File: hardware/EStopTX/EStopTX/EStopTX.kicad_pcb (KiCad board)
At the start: 2 copper layers, 75 x 59 mm, 11 parts

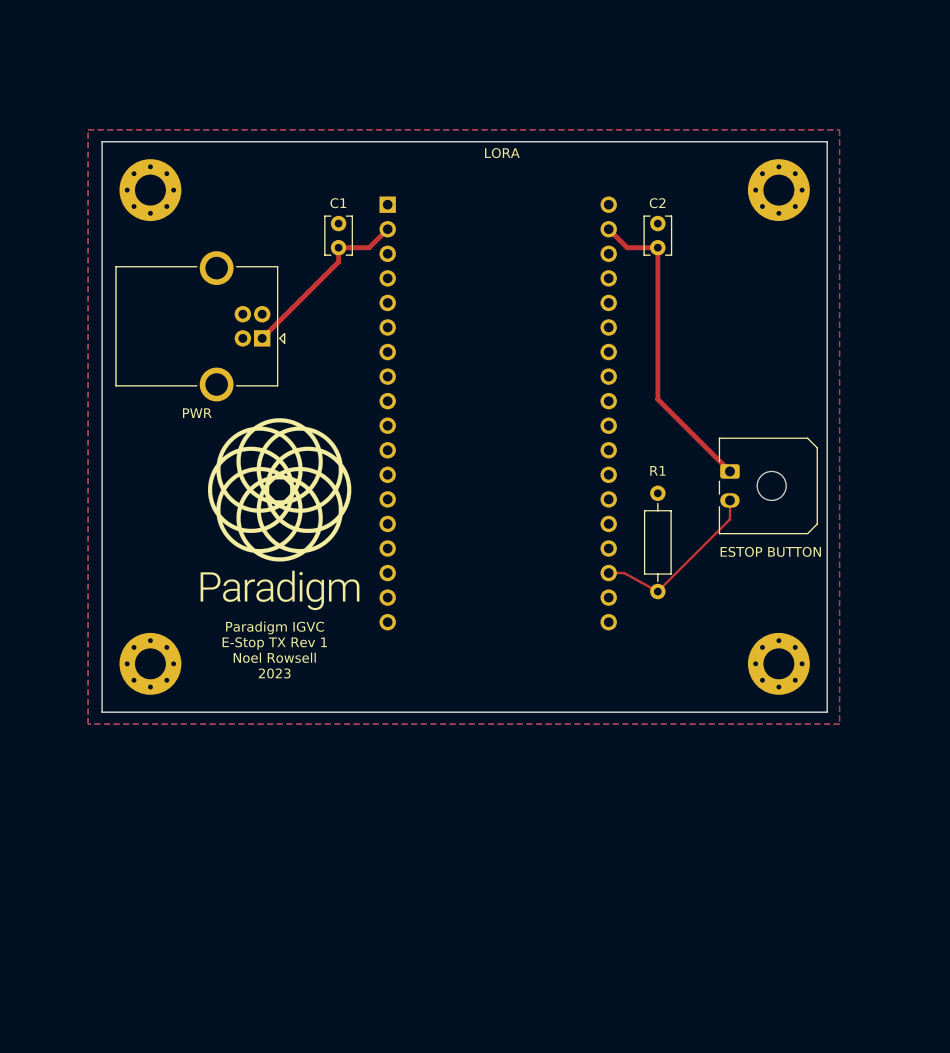
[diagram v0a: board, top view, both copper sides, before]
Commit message: adjustments
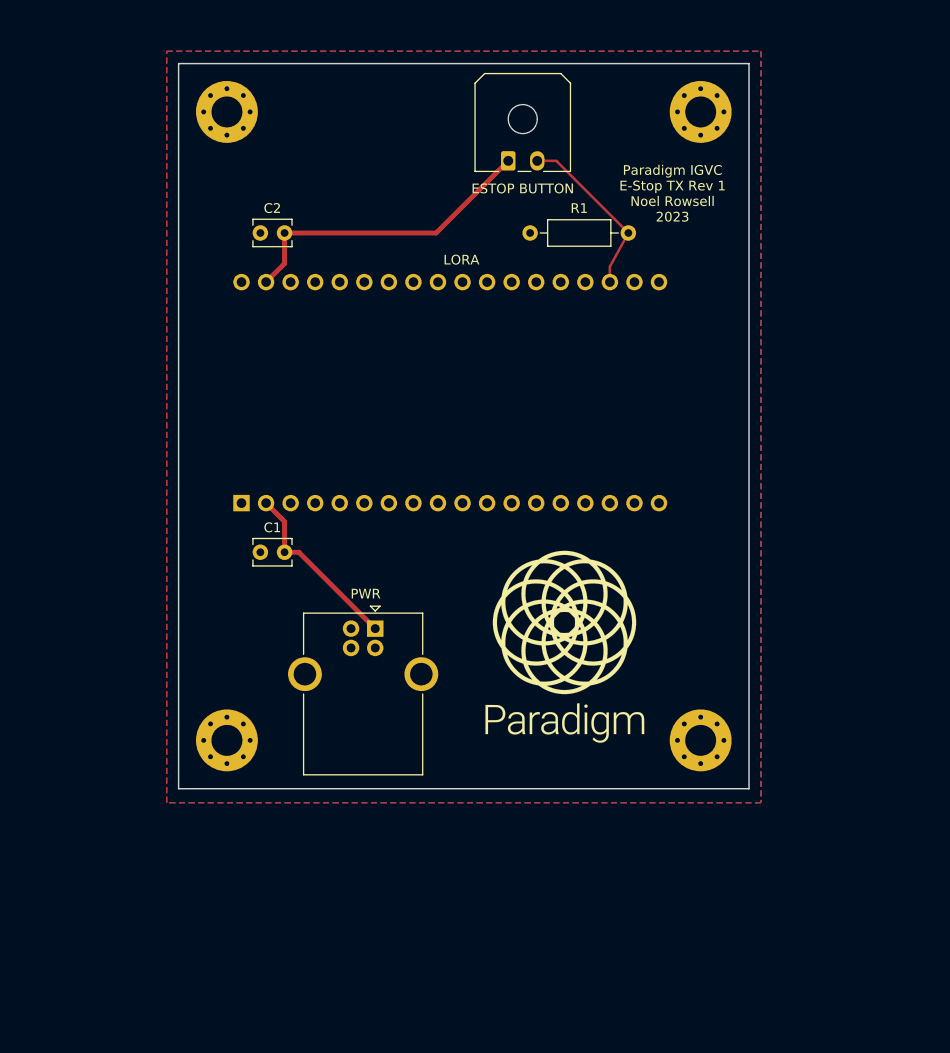
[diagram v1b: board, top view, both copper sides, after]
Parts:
- moved H2 57.7 mm to (112.9, 46.9), turned to 90 degrees
- moved H4 57.7 mm to (161.9, 46.9), turned to 90 degrees
- moved H1 57.5 mm to (112.9, 111.9), turned to 90 degrees
- moved H3 57.5 mm to (161.9, 111.9), turned to 90 degrees
- moved ESTOP BUTTON 39.5 mm to (142.0, 52.0), turned to 0 degrees
- moved C2 38.6 mm to (118.9, 59.4), turned to 180 degrees
- moved R1 37.2 mm to (154.4, 59.4), turned to 180 degrees
- moved C1 34.9 mm to (116.4, 92.5), turned to 0 degrees
- moved LORA 34.4 mm to (114.4, 87.4), turned to 90 degrees
- moved G*** 32.5 mm to (147.8, 102.4)
- moved PWR 32.2 mm to (128.2, 100.4), turned to -90 degrees
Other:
- board size 75 x 59 mm -> 59 x 75 mm

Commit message: changes
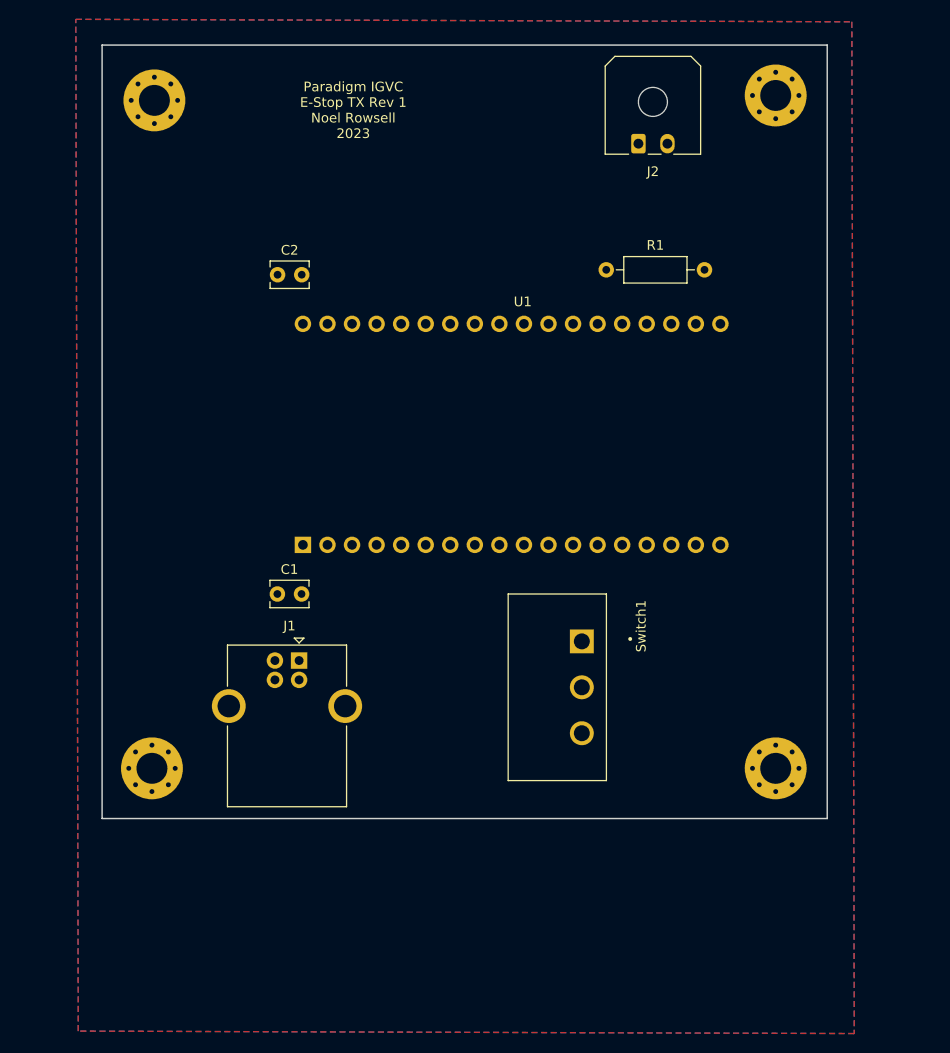
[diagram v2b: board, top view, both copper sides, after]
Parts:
- removed G***: LOGO, EStopFootprints:Paradigm_NameBelow_25.4mm
- added Switch1: L102021ML04Q, EStopFootprints:SW_L102021ML04Q, F.Cu at (149.6, 106.4)
- J2: renamed from ESTOP BUTTON
- moved J2 13.6 mm to (155.5, 50.2)
- moved R1 8.75 mm to (162.3, 63.2)
- moved J1 8.54 mm to (120.4, 103.7)
- moved H3 8.28 mm to (169.7, 114.8)
- moved H1 8.28 mm to (105.2, 114.8)
- moved H4 7.94 mm to (169.7, 45.2)
- moved U1 7.68 mm to (120.8, 91.7)
- moved H2 7.60 mm to (105.4, 45.7)
- moved C2 4.67 mm to (120.7, 63.8)
- moved C1 4.66 mm to (118.1, 96.8)
- renumbered PWR to J1, LORA to U1
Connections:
- J1 pad 1: +5V -> Net-(J1-Pad1)
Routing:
- net +5V: track 50.6 -> 0.00 mm
- net Net-(J2-Pad2): track 18.1 -> 0.00 mm
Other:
- board size 59 x 75 mm -> 75 x 80 mm

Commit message: hopefully done
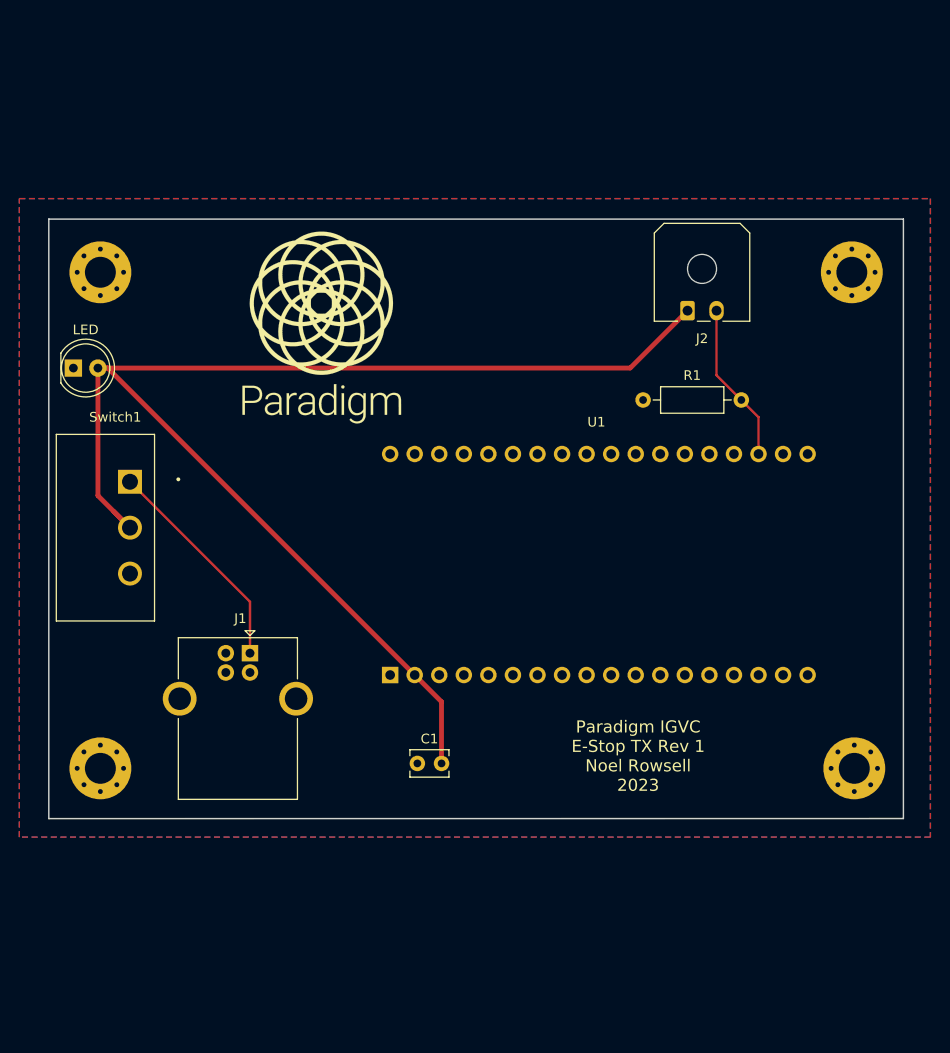
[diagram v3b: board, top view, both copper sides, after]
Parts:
- removed C2: 100n, Capacitor_THT:C_Disc_D3.8mm_W2.6mm_P2.50mm
- added G***: LOGO, EStopFootprints:Paradigm_NameBelow_25.4mm, F.Cu at (122.7, 69.3)
- added LED: LED, LED_THT:LED_D5.0mm, F.Cu at (97.0, 73.4)
- moved Switch1 49.6 mm to (102.9, 89.9)
- moved C1 22.7 mm to (132.6, 114.3)
- moved H4 19.9 mm to (177.5, 63.5)
- moved H2 18.6 mm to (99.8, 63.5)
- moved J2 18.0 mm to (160.6, 67.5)
- moved U1 16.2 mm to (129.8, 105.2)
- moved R1 14.0 mm to (166.1, 76.7)
- moved H3 8.13 mm to (177.8, 114.8)
- moved H1 5.33 mm to (99.8, 114.8)
- moved J1 5.14 mm to (115.3, 102.9)
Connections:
- U1 pad 20: +5V -> unconnected-(U1-Pad20)
- U1 pad 4: GND -> unconnected-(U1-Pad4)
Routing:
- net +5V: track 0.00 -> 139.9 mm
- net Net-(J1-Pad1): track 0.00 -> 22.9 mm
- net Net-(J2-Pad2): track 0.00 -> 16.6 mm
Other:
- board size 75 x 80 mm -> 88.4 x 62 mm
